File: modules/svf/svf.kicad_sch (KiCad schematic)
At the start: 35 parts, among them U1 VTL5C, U2 VTL5C, U3 MCP6002-xSN, U4 MCP6002-xSN, U5 MCP6002-xSN

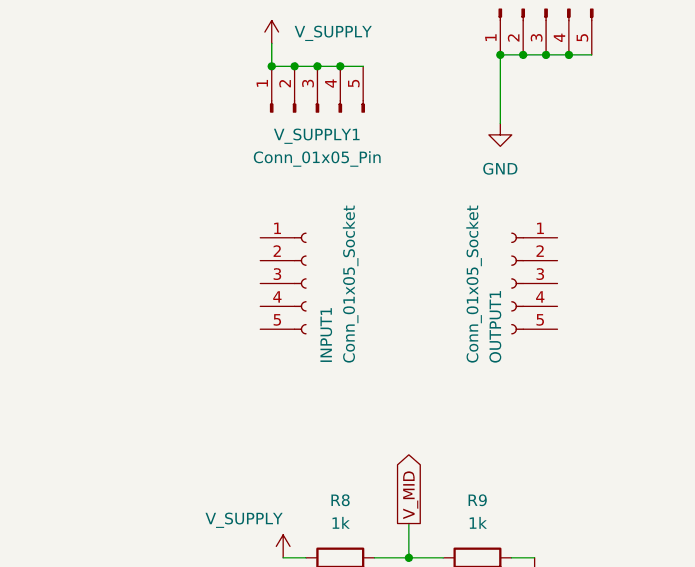
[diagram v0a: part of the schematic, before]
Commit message: Getting it ready for PCB routing
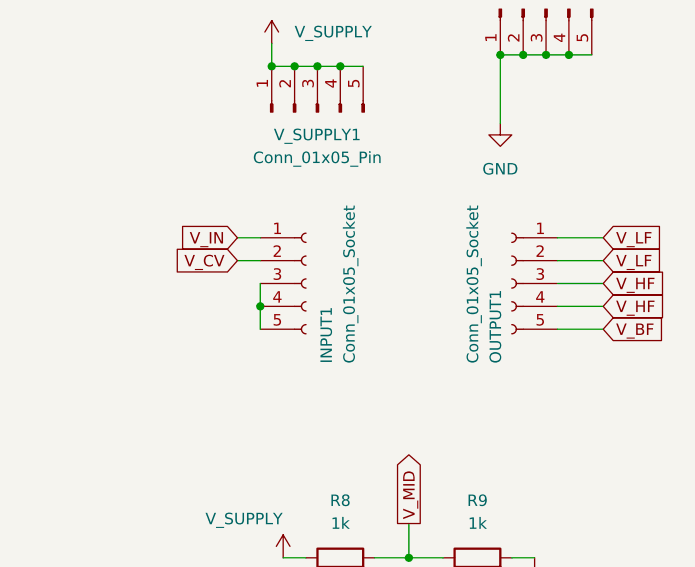
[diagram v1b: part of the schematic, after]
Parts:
- C1, C2, C3, C4, C5: footprint (none) -> Capacitor_SMD:C_0402_1005Metric
- R1, R10, R11, R12, R13, R14, R15, R16, R2, R3, R4, R5, R6, R7, R8, R9: footprint (none) -> Resistor_SMD:R_0402_1005Metric
- RV1, RV2: footprint (none) -> BreadModular_Pots:Potentiometer_RV09
- U3, U4, U5: footprint (none) -> Package_SO:SOIC-8-1EP_3.9x4.9mm_P1.27mm_EP2.29x3mm
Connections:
- net V_BF: now also OUTPUT1.5 (Pin_5)
- net V_CV: now also INPUT1.2 (Pin_2)
- net V_HF: now also OUTPUT1.3 (Pin_3), OUTPUT1.4 (Pin_4)
- net V_IN: now also INPUT1.1 (Pin_1)
- net V_LF: now also OUTPUT1.1 (Pin_1), OUTPUT1.2 (Pin_2)
- net at INPUT1.3 (Pin_3): now also INPUT1.4 (Pin_4), INPUT1.5 (Pin_5)
